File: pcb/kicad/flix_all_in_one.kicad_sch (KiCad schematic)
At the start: 14 parts, among them J1 UJ20-C-H-G-MSMT-2B-P16-TR, J2 BM03B-GHS-TBT_LF__SN__N_, J3 BM02B-GHS-TBT_LF__SN__N_, J4 BM02B-GHS-TBT_LF__SN__N_, J5 BM02B-GHS-TBT_LF__SN__N_, J6 BM02B-GHS-TBT_LF__SN__N_, U3 TP4054ST25P, U4 ME6211C33M5

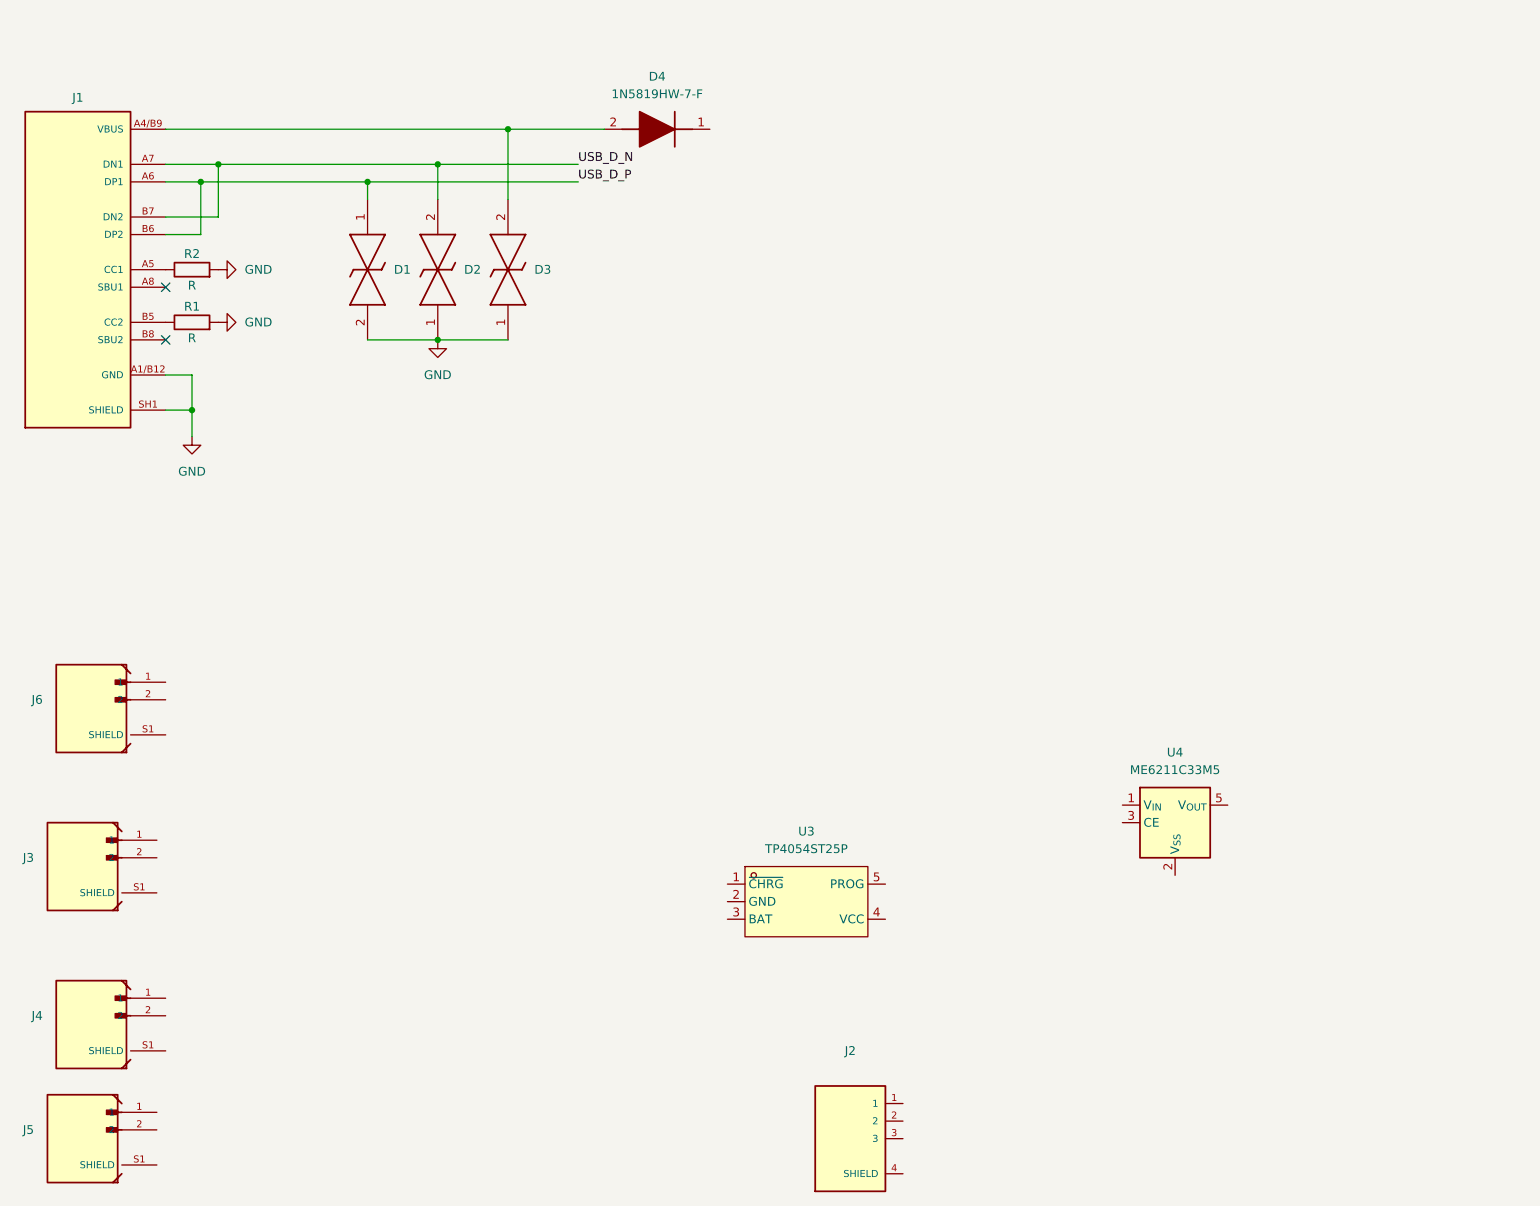
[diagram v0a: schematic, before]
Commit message: update libs and sch
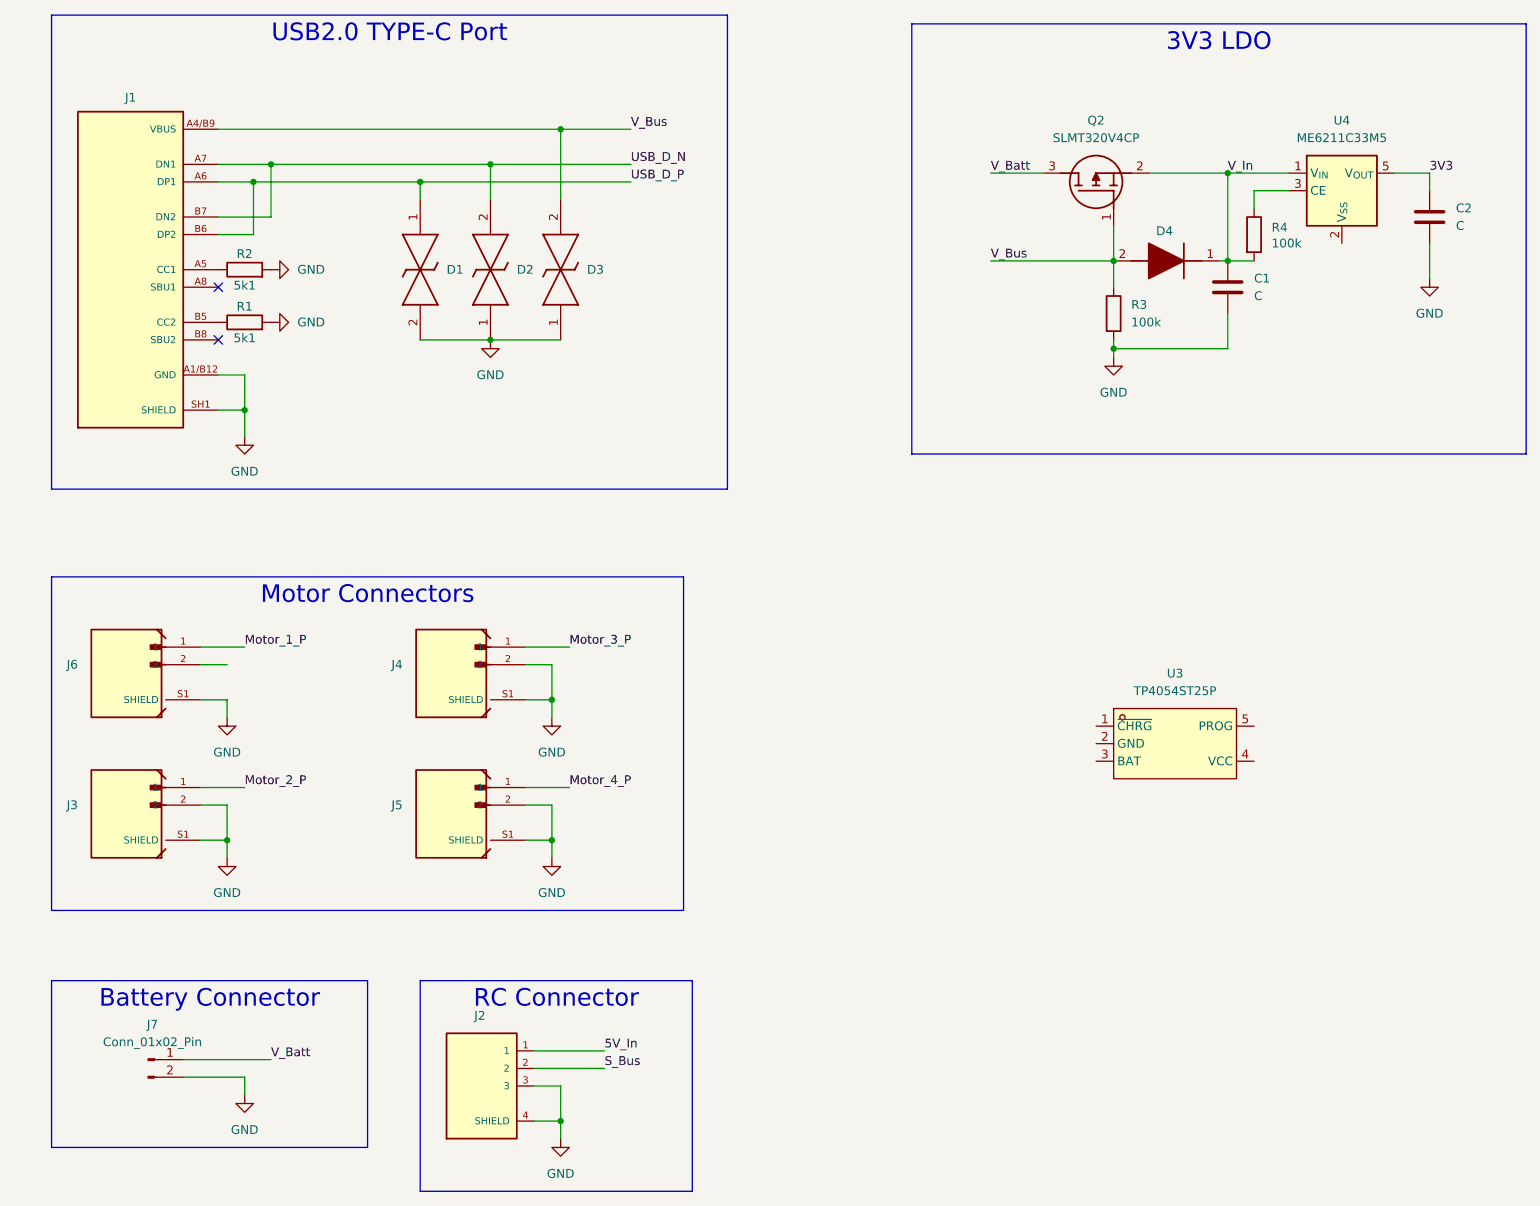
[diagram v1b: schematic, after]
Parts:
- added C1, C2: C, symbol Device:C
- added J7: Conn_01x02_Pin, symbol Connector:Conn_01x02_Pin
- added Q2: SLMT320V4CP, SOT95P280X110-3N, symbol SLMT320V4CP:SLMT320V4CP
- added R3, R4: 100k, symbol Device:R
- R1, R2: value R -> 5k1
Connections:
- net GND: now also J2.3, J2.4 (SHIELD), J2.5 (SHIELD), J3.2, J3.S1 (SHIELD), J3.S2 (SHIELD), J4.2, J4.S1 (SHIELD), J4.S2 (SHIELD), J5.2, J5.S1 (SHIELD), J5.S2 (SHIELD), J6.S1 (SHIELD), J6.S2 (SHIELD), C1.2, C2.2, J7.2 (Pin_2), R3.2
- net VBUS: now also Q2.1 (G), R3.1
- net Motor_4_P: now reaches J5.1
- net V_In: now reaches D4.1 (K)
- net V_In: now also U4.1 (V_{IN}), C1.1, Q2.2 (S), R4.2
- net Motor_3_P: now reaches J4.1
- net Motor_2_P: now reaches J3.1
- net 5V_In: now reaches J2.1
- net S_Bus: now reaches J2.2
- net Motor_1_P: now reaches J6.1
- net at U4.3 (CE): now also R4.1
- net 3V3: now reaches U4.5 (V_{OUT})
- net 3V3: now also C2.1
- new net V_Batt: J7.1 (Pin_1), Q2.3 (D)
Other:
- moved on the sheet: D1, D2, D3, D4, J1, J2, J3, J4, J5, J6, R1, R2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
